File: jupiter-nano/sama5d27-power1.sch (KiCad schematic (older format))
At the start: 45 parts, among them U1 ATSAMA5D27C-LD1G-CU

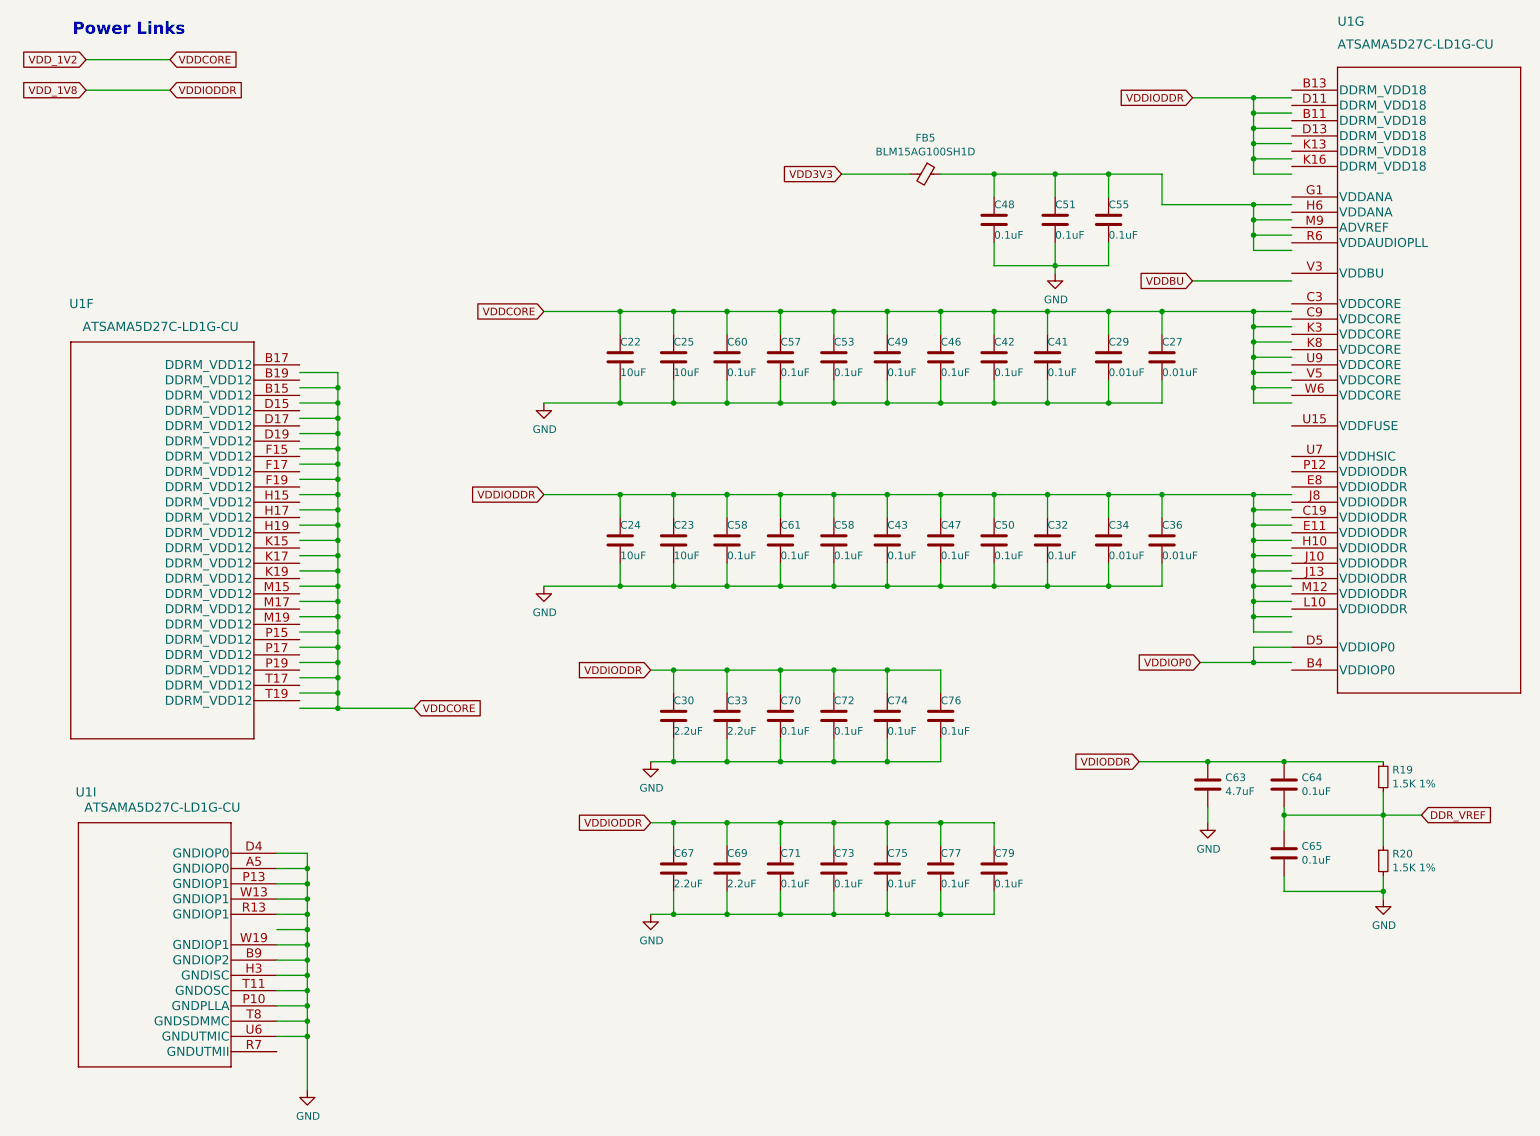
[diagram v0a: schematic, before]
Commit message: WIP, power done
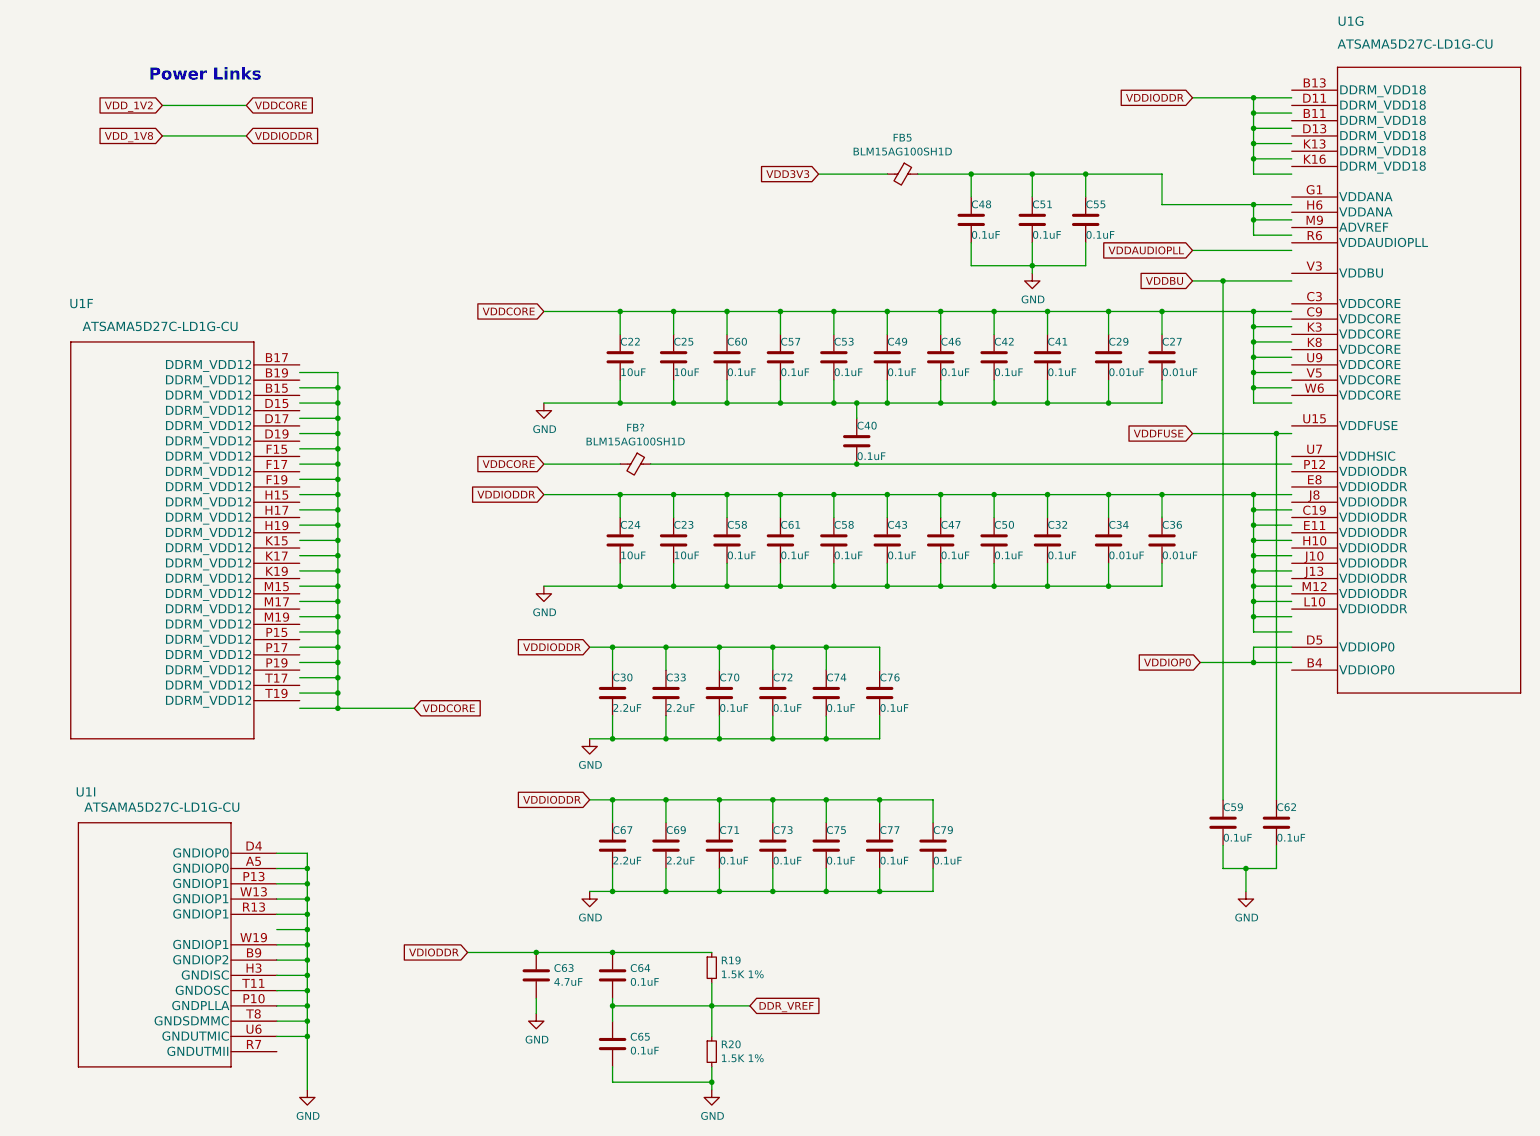
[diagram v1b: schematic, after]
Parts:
- added C40, C59, C62: 0.1uF, symbol Device:C
- added FB?: BLM15AG100SH1D, Capacitor_SMD:C_0402_1005Metric, symbol Device:Ferrite_Bead_Small
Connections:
- net labels added: VDDAUDIOPLL, VDDFUSE
- wire segments 302 -> 316
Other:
- moved on the sheet: C30, C33, C48, C51, C55, C63, C64, C65, C67, C69, C70, C71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
